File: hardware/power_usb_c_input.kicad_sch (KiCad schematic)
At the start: 38 parts, among them J1 DX07S024JJ2R1300, Q1 AGM612AP, Q2 AO3404A, U1 TPD4S480RUKR

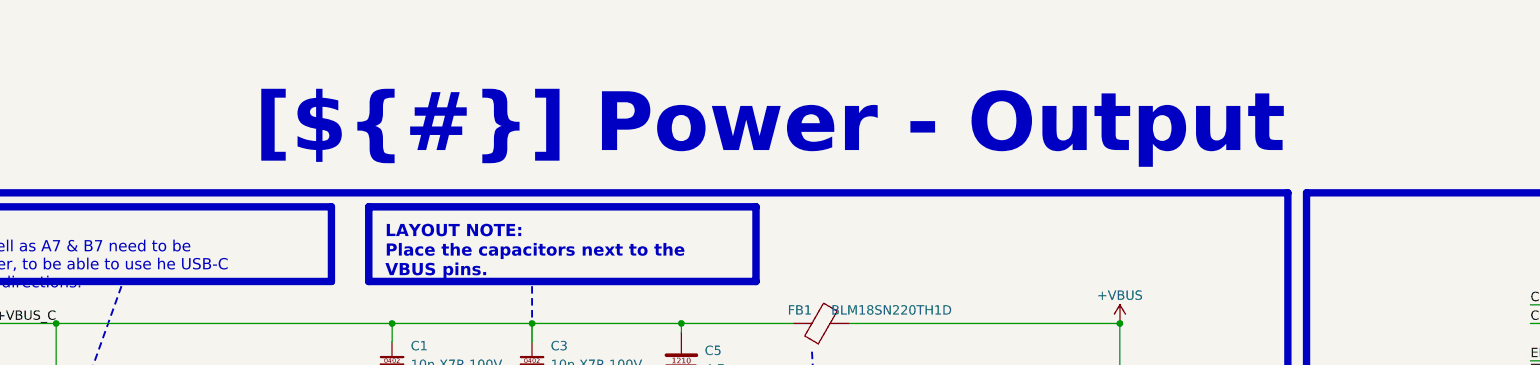
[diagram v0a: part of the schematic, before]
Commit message: Generate hardware documentation
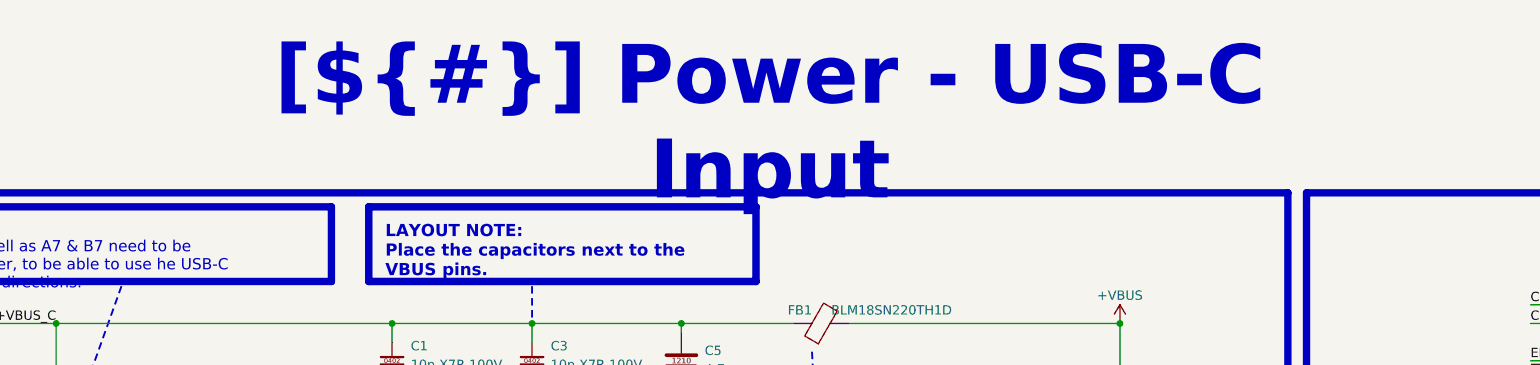
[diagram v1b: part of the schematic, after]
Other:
- title: Power - Output -> Power - USB-C Input
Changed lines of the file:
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@@
 	(paper "A3")
 	(title_block
-		(title "Power - Output")
+		(title "Power - USB-C Input")
 		(date "2026-02-27")
 		(rev "${REVISION}")
